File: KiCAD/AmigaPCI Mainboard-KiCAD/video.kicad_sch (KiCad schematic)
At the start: 51 parts, among them CN300 DB15_Female_HighDensity, CN301 Video-Slot, CN302 Video-Slot, CN303 Raspberry_Pi_Zero, J301 PI_BUTTON, J303 HSYNC/COMPSYNC, U201 74LVC1G74, U300 DENISE, U301 74AHCT244, U302 74AHCT244, U303 74LVC574, U304 74LVC574, U305 74HCT08, U307 74LVC86

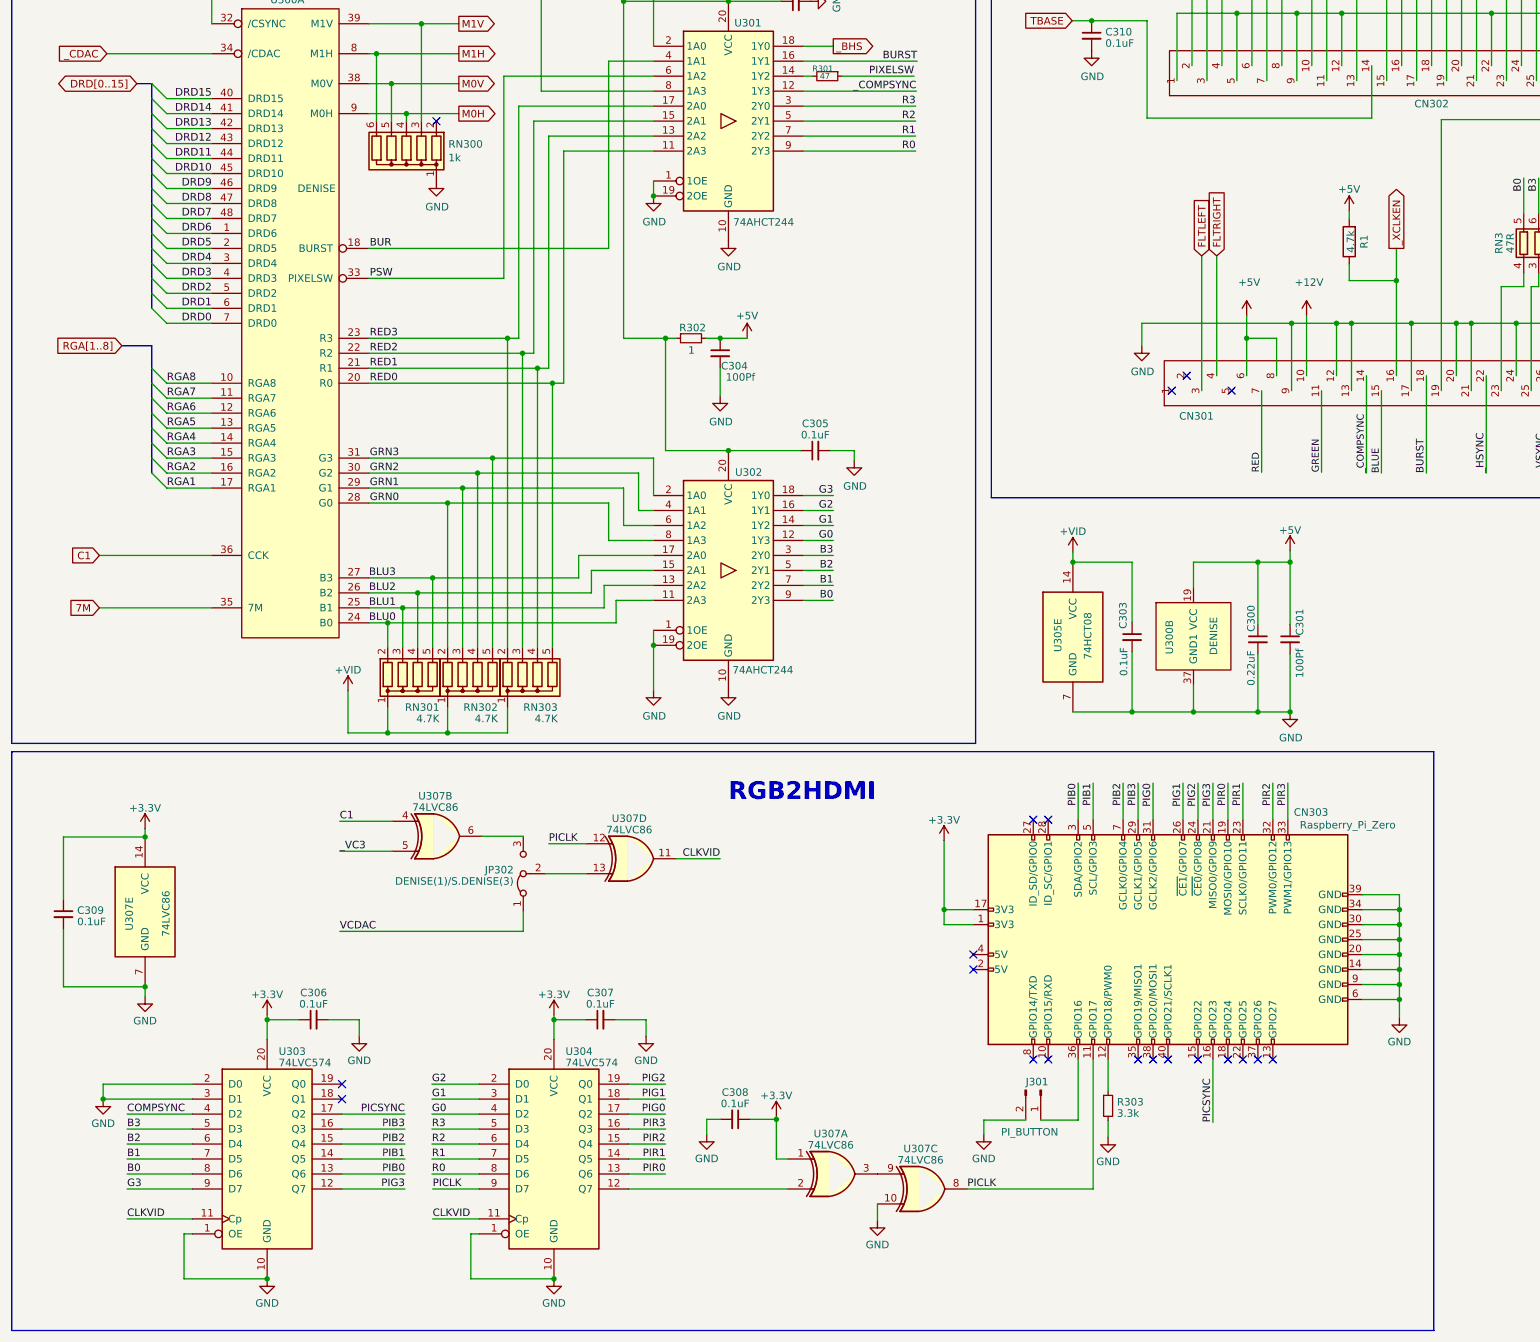
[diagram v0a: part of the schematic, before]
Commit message: Routing June 10 2023b
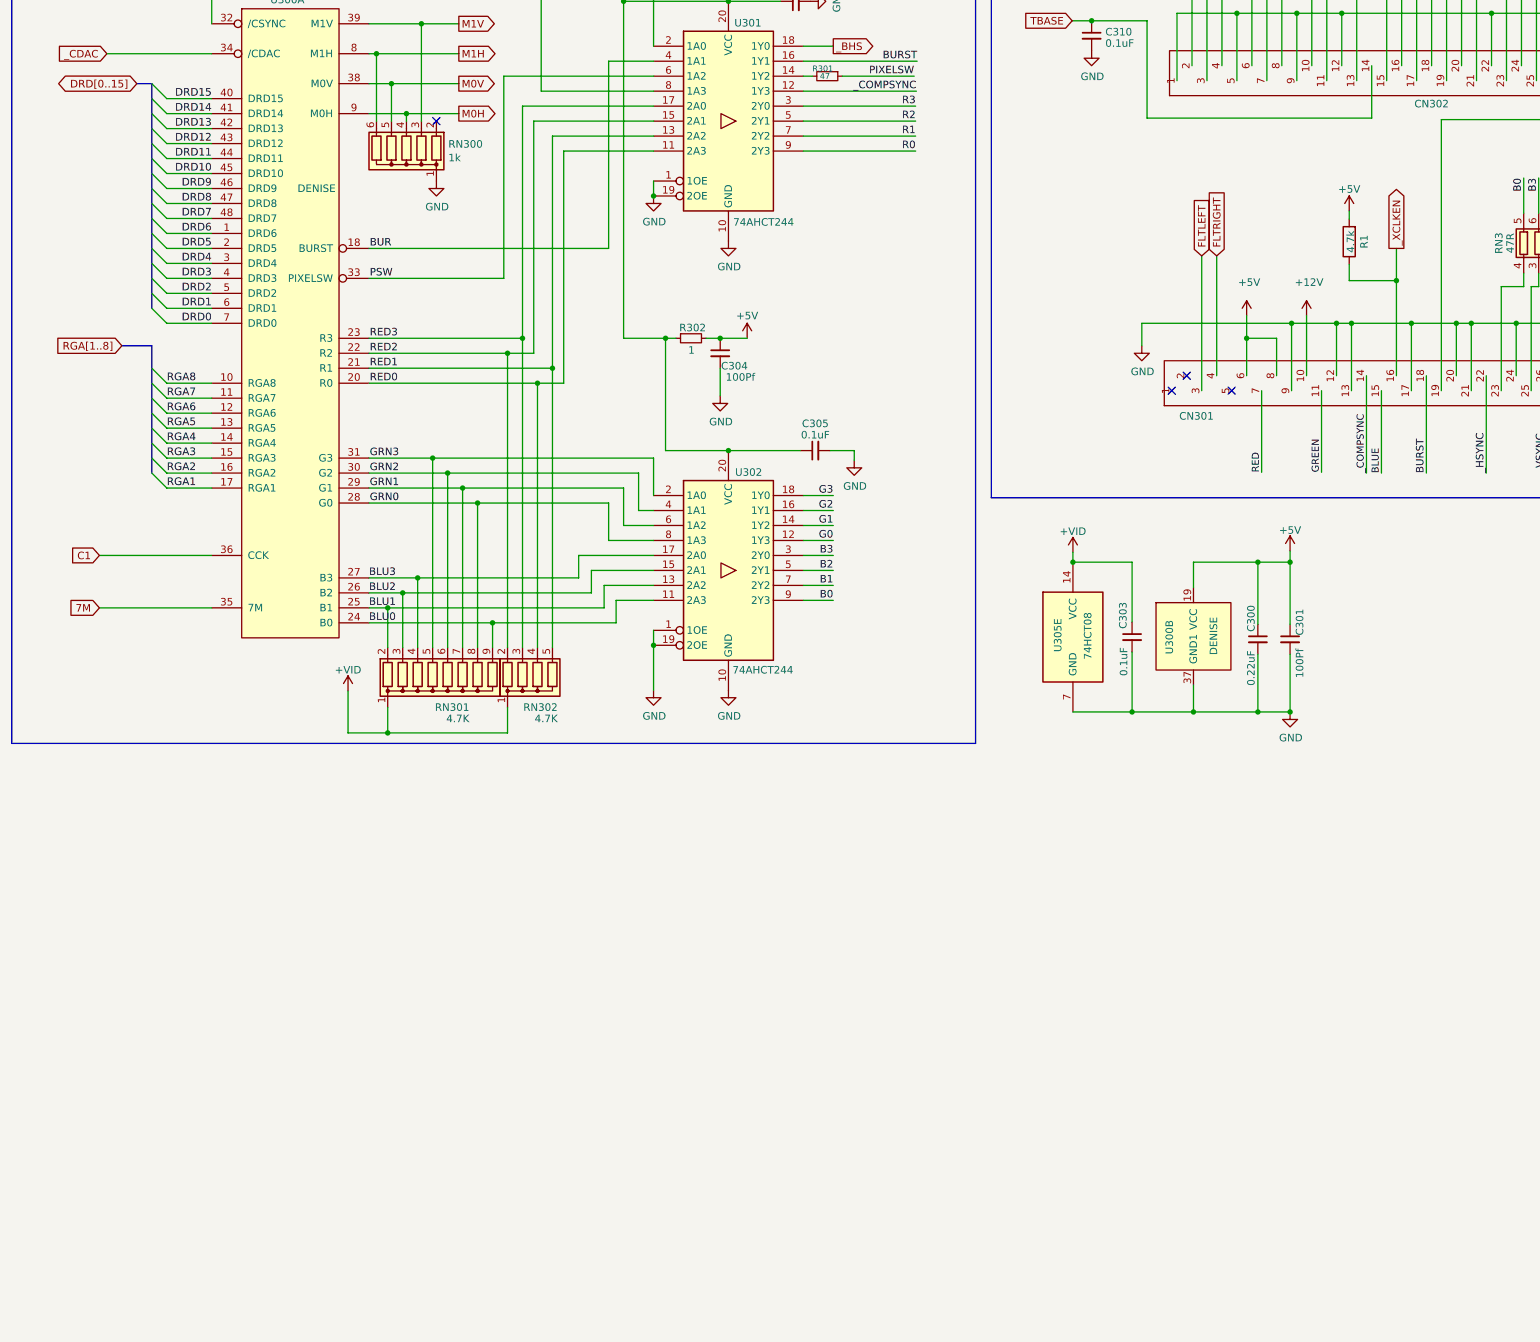
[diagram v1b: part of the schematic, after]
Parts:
- removed C306, C307, C308, C309: 0.1uF, Capacitor_SMD:C_0603_1608Metric, symbol Device:C_Small
- removed CN303: Raspberry_Pi_Zero, Connector_PinSocket_2.54mm:PinSocket_2x20_P2.54mm_Vertical, symbol Connector:Raspberry_Pi_2_3
- removed J301: PI_BUTTON, Connector_PinHeader_2.54mm:PinHeader_1x02_P2.54mm_Vertical, symbol Connector:Conn_01x02_Pin
- removed JP302: DENISE(1)/S.DENISE(3), Connector_PinHeader_2.54mm:PinHeader_1x03_P2.54mm_Vertical, symbol Jumper:Jumper_3_Bridged12
- removed R303: 3.3k, Resistor_SMD:R_0603_1608Metric, symbol Device:R_Small
- removed RN302: 4.7K, Resistor_THT:R_Array_SIP5, symbol Device:R_Network04
- removed U303, U304: 74LVC574, Package_SO:TSSOP-20_4.4x6.5mm_P0.65mm, symbol 74xx:74LS574
- removed U307: 74LVC86, Package_SO:TSSOP-14_4.4x5mm_P0.65mm, symbol 74xx:74LS86
- RN301: footprint Resistor_THT:R_Array_SIP5 -> Resistor_THT:R_Array_SIP9; symbol Device:R_Network04 -> Device:R_Network08
- renumbered RN303 to RN302
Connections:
- net BLU0: now also RN301.9 (R8); no longer RN301.2 (R1)
- net BLU1: now also RN301.2 (R1); no longer RN301.3 (R2)
- net BLU2: now also RN301.3 (R2); no longer RN301.4 (R3)
- net BLU3: now also RN301.4 (R3); no longer RN301.5 (R4)
- net GRN0: now also RN301.8 (R7)
- net GRN1: now also RN301.7 (R6)
- net GRN2: now also RN301.6 (R5)
- net GRN3: now also RN301.5 (R4)
- net RED0: now also RN302.4 (R3); no longer RN302.5 (R4)
- net RED1: now also RN302.5 (R4); no longer RN302.4 (R3)
- net RED2: now also RN302.2 (R1); no longer RN302.3 (R2)
- net RED3: now also RN302.3 (R2); no longer RN302.2 (R1)
- no-connect marks 27 -> 11
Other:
- note removed: "RGB2HDMI"
